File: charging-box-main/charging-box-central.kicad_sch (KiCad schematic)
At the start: 24 parts, among them J1 Accumulator 1, J10 mains power indicator, J11 Close AIRs, J2 Accumulator 2, J3 Main 12V, J4 Latching, J5 Charger, J6 IMD FAULT LED active low, J7 BMS LED active low, J8 Latching reset, J9 JESUS button, SW11 ON BUTTON

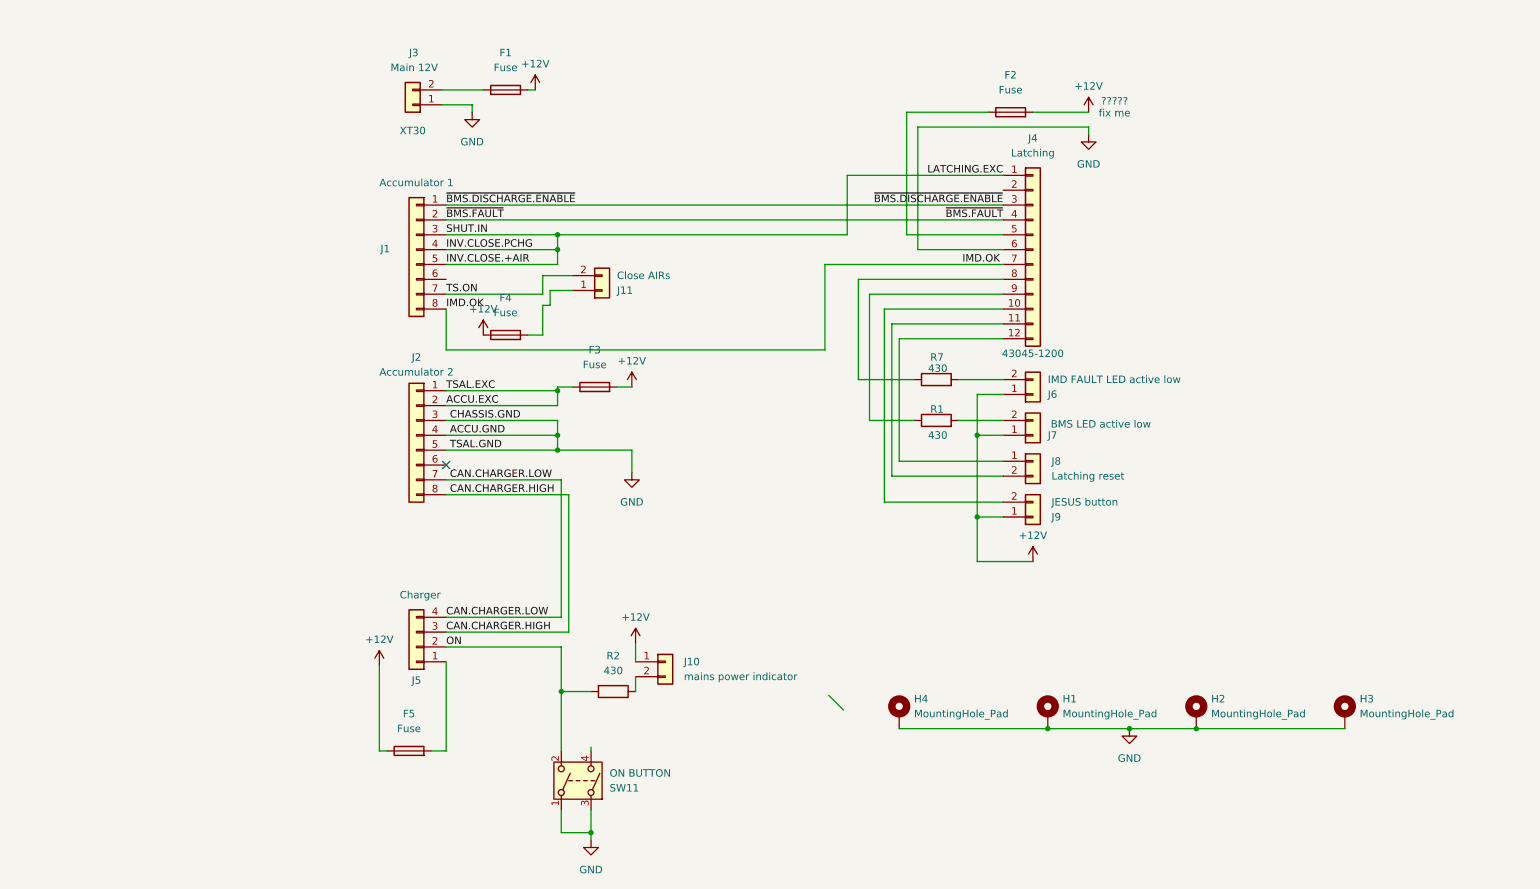
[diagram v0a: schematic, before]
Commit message: made it a lill bit neater
not much
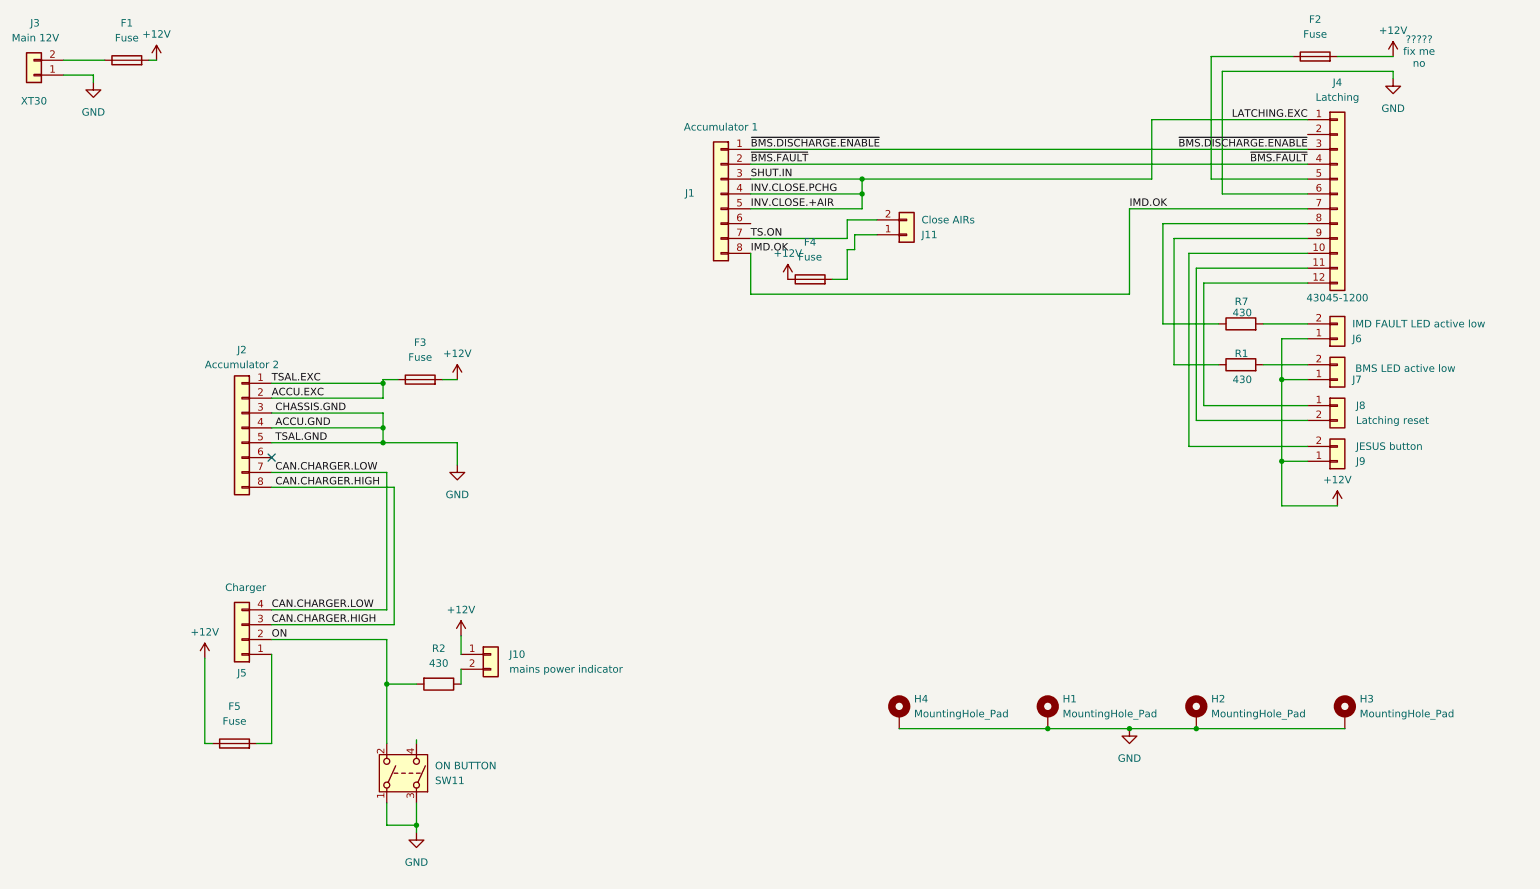
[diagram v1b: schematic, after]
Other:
- note added: "????? fix me no"
- note removed: "????? fix me"
- moved on the sheet: F1, F2, F3, F4, F5, J1, J10, J11, J2, J3, J4, J5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
